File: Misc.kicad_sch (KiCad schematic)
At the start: 24 parts, among them J501 Conn_01x04, J502 TE 338069-4, J503 Conn_01x10, J504 Conn_01x10, J505 Conn_01x10, J506 Conn_01x10, J507 Conn_02x05_Odd_Even, J508 Conn_02x05_Odd_Even, J509 Conn_01x05, J510 Conn_01x05, U501 SN65HVD232QDRQ1, U502 TXS0102DCU

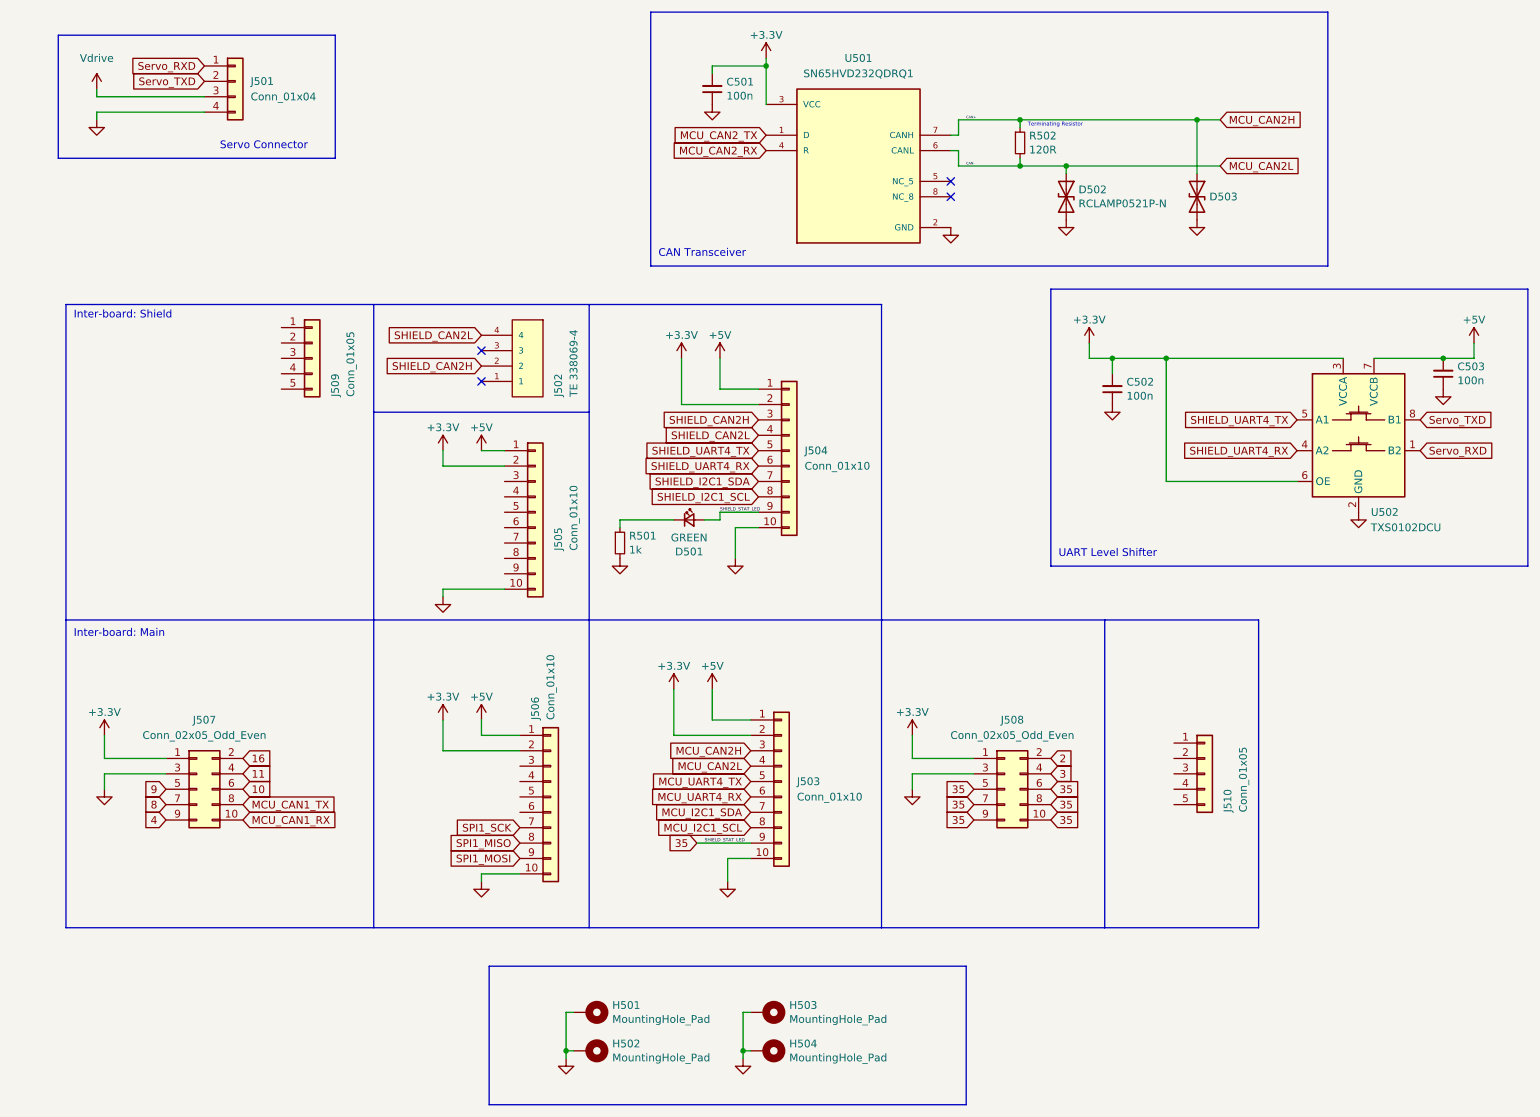
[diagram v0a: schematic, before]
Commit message: sdgnseiogniosegn
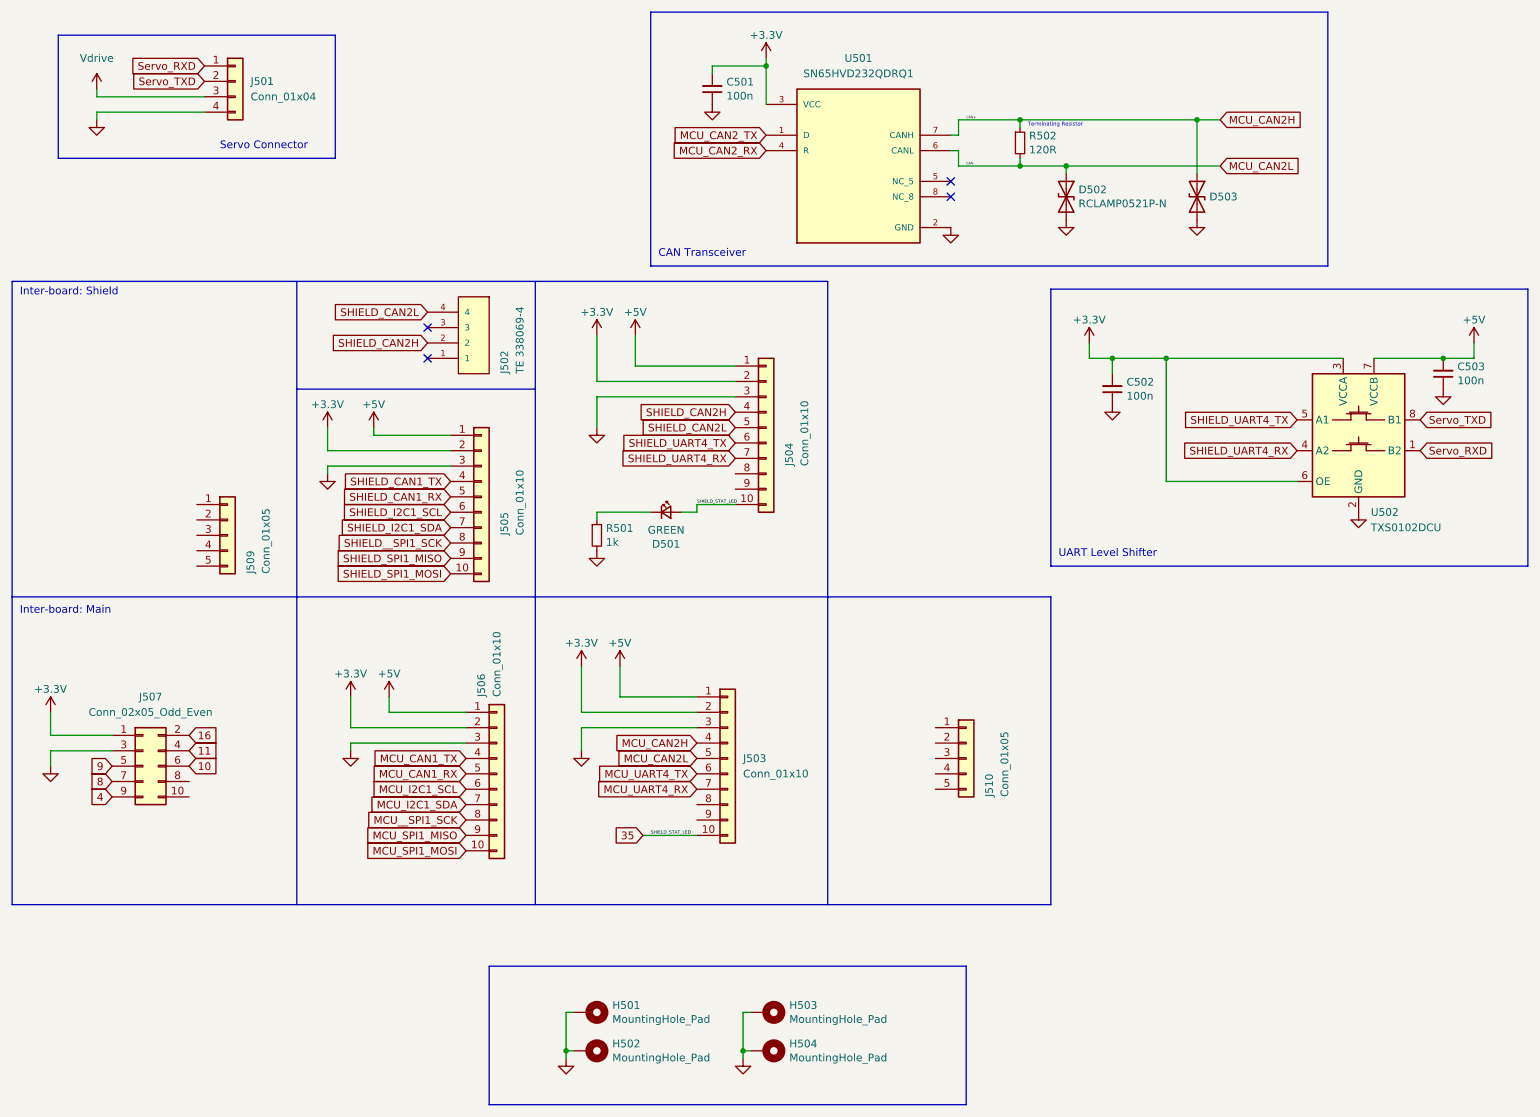
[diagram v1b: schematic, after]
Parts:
- removed J508: Conn_02x05_Odd_Even, Connector_PinSocket_2.54mm:PinSocket_2x05_P2.54mm_Vertical, symbol Connector_Generic:Conn_02x05_Odd_Even
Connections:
- net SPI1_SCK is gone; now on net MCU_I2C1_SDA: J506.7 (Pin_7)
- net 35: now also J503.10 (Pin_10), J504.10 (Pin_10); no longer J503.9 (Pin_9), J504.9 (Pin_9)
- net GND: now also J503.3 (Pin_3), J504.3 (Pin_3), J505.3 (Pin_3), J506.3 (Pin_3); no longer J503.10 (Pin_10), J504.10 (Pin_10), J505.10 (Pin_10), J506.10 (Pin_10)
- net MCU_CAN1_RX: now also J506.5 (Pin_5); no longer J507.10 (Pin_10)
- net MCU_CAN1_TX: now also J506.4 (Pin_4); no longer J507.8 (Pin_8)
- net MCU_CAN2H: now also J503.4 (Pin_4); no longer J503.3 (Pin_3)
- net MCU_CAN2L: now also J503.5 (Pin_5); no longer J503.4 (Pin_4)
- net MCU_I2C1_SCL: now also J506.6 (Pin_6); no longer J503.8 (Pin_8)
- net MCU_I2C1_SDA: no longer J503.7 (Pin_7)
- net MCU_UART4_RX: now also J503.7 (Pin_7); no longer J503.6 (Pin_6)
- net MCU_UART4_TX: now also J503.6 (Pin_6); no longer J503.5 (Pin_5)
- net SHIELD_CAN2H: now also J504.4 (Pin_4); no longer J504.3 (Pin_3)
- net SHIELD_CAN2L: now also J504.5 (Pin_5); no longer J504.4 (Pin_4)
- net SHIELD_I2C1_SCL: now also J505.6 (Pin_6); no longer J504.8 (Pin_8)
- net SHIELD_I2C1_SDA: now also J505.7 (Pin_7); no longer J504.7 (Pin_7)
- net SHIELD_UART4_RX: now also J504.7 (Pin_7); no longer J504.6 (Pin_6)
- net SHIELD_UART4_TX: now also J504.6 (Pin_6); no longer J504.5 (Pin_5)
- net SHIELD_CAN1_TX: now reaches J505.4 (Pin_4)
- net SHIELD_CAN1_RX: now reaches J505.5 (Pin_5)
- net SHIELD__SPI1_SCK: now reaches J505.8 (Pin_8)
- net SHIELD_SPI1_MISO: now reaches J505.9 (Pin_9)
- net SPI1_MISO renamed MCU__SPI1_SCK
- net SPI1_MOSI renamed MCU_SPI1_MISO
- new net MCU_SPI1_MOSI: J506.10 (Pin_10)
- new net SHIELD_SPI1_MOSI: J505.10 (Pin_10)
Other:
- moved on the sheet: J502, J503, J504, J505, J506, J507, J509, J510

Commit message: oenbioernb
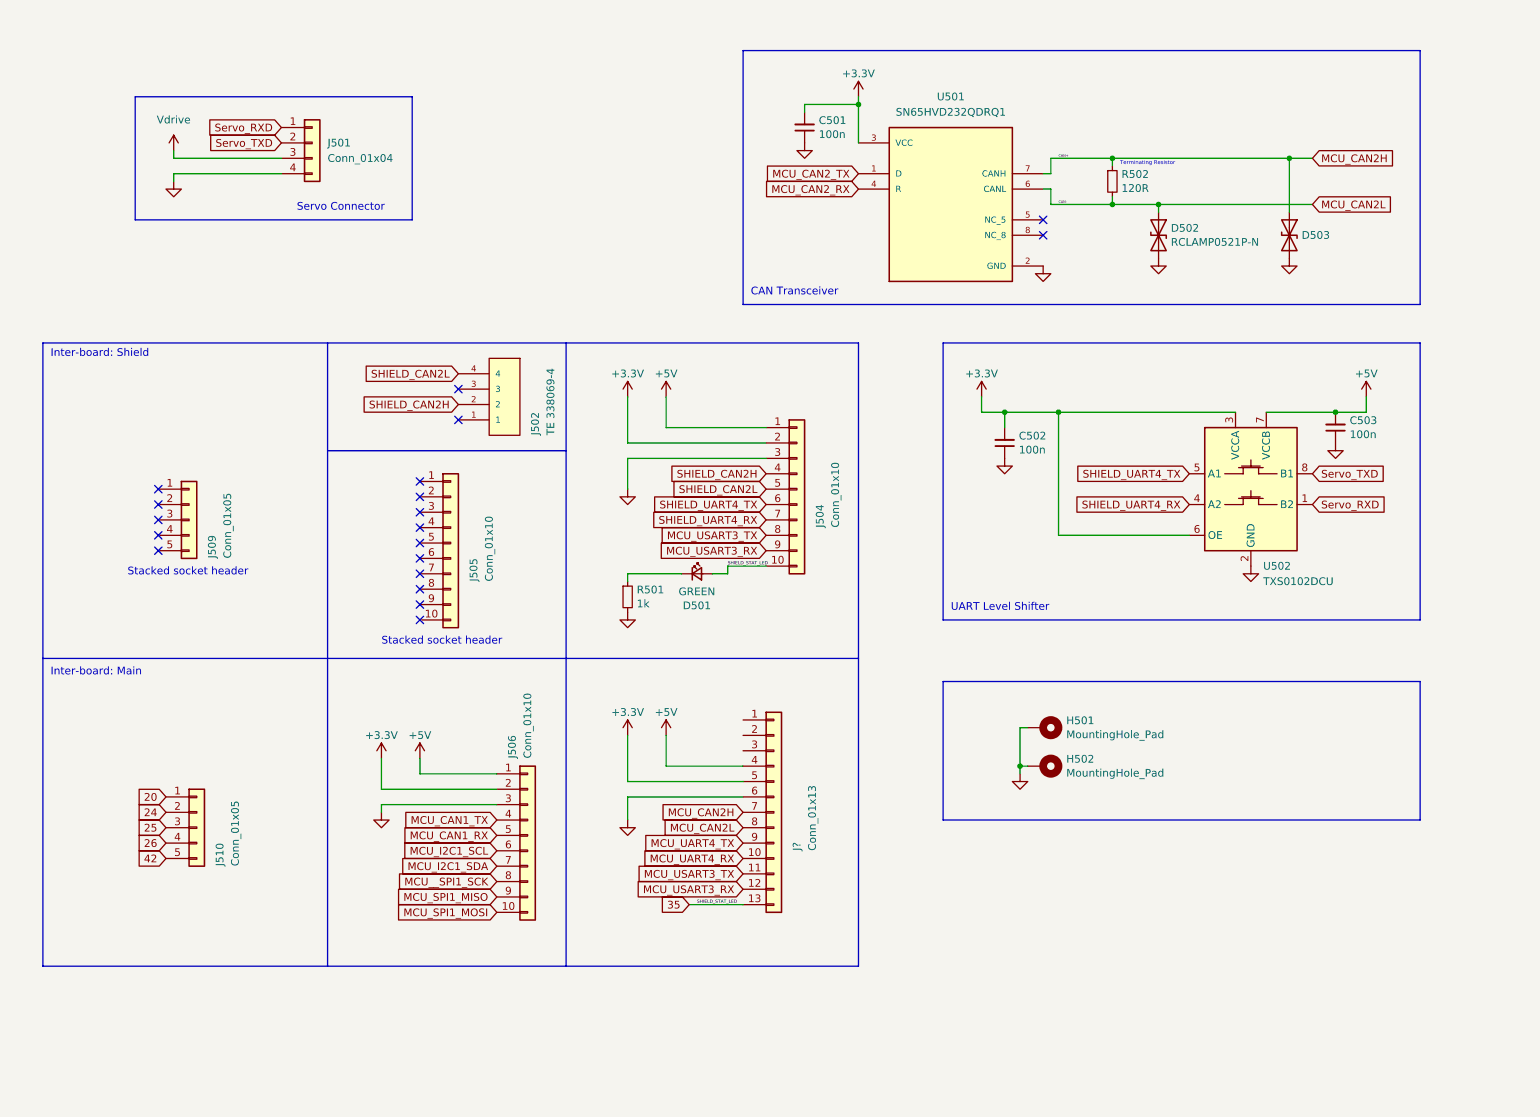
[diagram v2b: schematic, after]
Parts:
- removed H502, H504: MountingHole_Pad, MountingHole:MountingHole_3.2mm_M3_Pad_Via, symbol Mechanical:MountingHole_Pad
- removed J503: Conn_01x10, Connector_PinSocket_2.54mm:PinSocket_1x10_P2.54mm_Vertical, symbol Connector_Generic:Conn_01x10
- removed J507: Conn_02x05_Odd_Even, Connector_PinSocket_2.54mm:PinSocket_2x05_P2.54mm_Vertical, symbol Connector_Generic:Conn_02x05_Odd_Even
- added J?: Conn_01x13, symbol Connector_Generic:Conn_01x13
- renumbered H503 to H502
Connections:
- net +3V3: now also J?.5 (Pin_5); no longer J505.2 (Pin_2)
- net +5V: now also J?.4 (Pin_4); no longer J505.1 (Pin_1)
- net 35: now also J?.13 (Pin_13)
- net GND: now also J?.6 (Pin_6); no longer J505.3 (Pin_3)
- net MCU_CAN2H: now also J?.7 (Pin_7)
- net MCU_CAN2L: now also J?.8 (Pin_8)
- net MCU_UART4_RX: now also J?.10 (Pin_10)
- net MCU_UART4_TX: now also J?.9 (Pin_9)
- net MCU_USART3_TX: now reaches J504.8 (Pin_8)
- net MCU_USART3_TX: now also J?.11 (Pin_11)
- net MCU_USART3_RX: now reaches J504.9 (Pin_9)
- net MCU_USART3_RX: now also J?.12 (Pin_12)
- net 20: now reaches J510.1 (Pin_1)
- net 24: now reaches J510.2 (Pin_2)
- net 25: now reaches J510.3 (Pin_3)
- net 26: now reaches J510.4 (Pin_4)
- net 42: now reaches J510.5 (Pin_5)
- net SHIELD_CAN1_RX: no longer names the net of J505.5 (Pin_5)
- net SHIELD_CAN1_TX: no longer names the net of J505.4 (Pin_4)
- net SHIELD_I2C1_SCL: no longer names the net of J505.6 (Pin_6)
- net SHIELD_I2C1_SDA: no longer names the net of J505.7 (Pin_7)
- net SHIELD_SPI1_MISO: no longer names the net of J505.9 (Pin_9)
- net SHIELD_SPI1_MOSI: no longer names the net of J505.10 (Pin_10)
- net SHIELD__SPI1_SCK: no longer names the net of J505.8 (Pin_8)
- no-connect marks 4 -> 19
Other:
- note added: "Stacked socket header"
- moved on the sheet: C501, C502, C503, D501, D502, D503, H501, H502, J501, J502, J504, J505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
